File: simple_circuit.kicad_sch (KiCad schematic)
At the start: 1 part

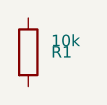
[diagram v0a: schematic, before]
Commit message: continue working claude setup
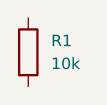
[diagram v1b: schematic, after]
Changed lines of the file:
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@@
 		(fields_autoplaced yes)
 		(property "Reference" "R1"
-			(at 102.54 100 0)
+			(at 102.54 98.73 0)
 			(effects
 				(font
@@
 				(justify left)))
 		(property "Value" "10k"
-			(at 102.54 98.73 0)
+			(at 102.54 101.27 0)
 			(effects
 				(font
 					(size 1.27 1.27))
-				(justify left))))
+				(justify left)))
+		(pin "1"
+)
+		(pin "2"
+)
+		(instances
+			(project "simple_circuit" (path "/9d4d9269-d775-4e3a-a2b9-d17cf97d721e" (reference "R1") (unit 1)))))
 	(symbol_instances))
